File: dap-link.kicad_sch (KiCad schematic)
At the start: 46 parts, among them J1 Molex 0473460001, J2 Conn_01x05_Male, J3 SWD 10 pin 2.54mm, J4 SWD 10 pin 1.27mm, Q1 MMBT3904, U1 SC573V33RTRC, U2 STM32F103CBTx, U3 150141SV73110, Y1 8MHz

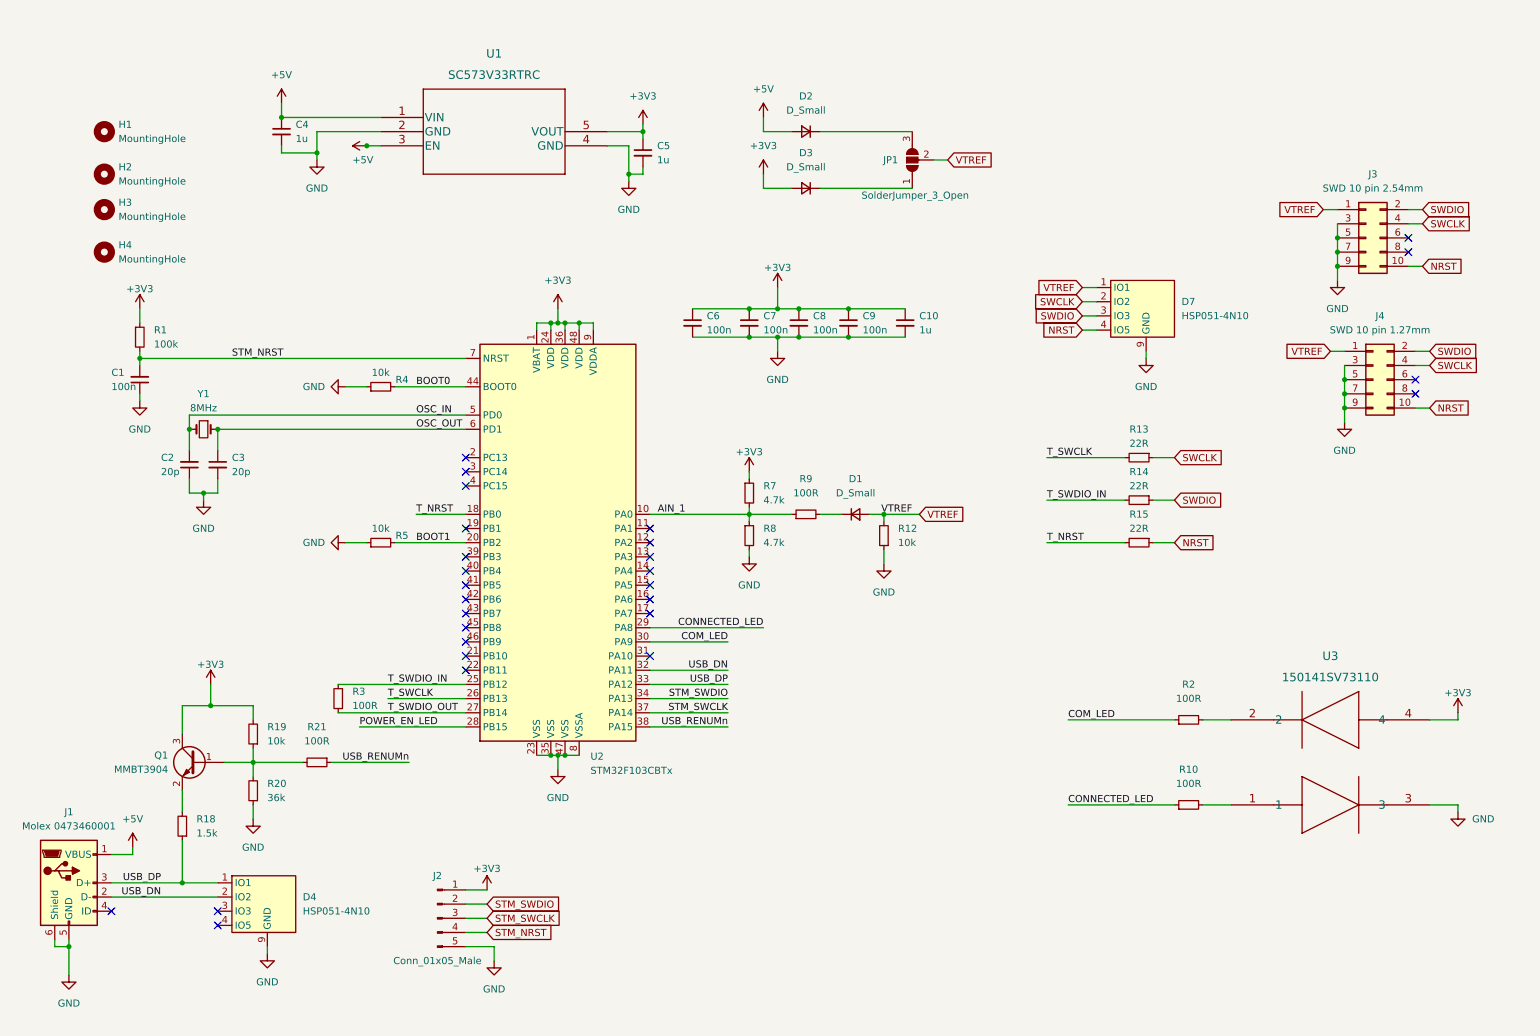
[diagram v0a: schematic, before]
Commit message: changes
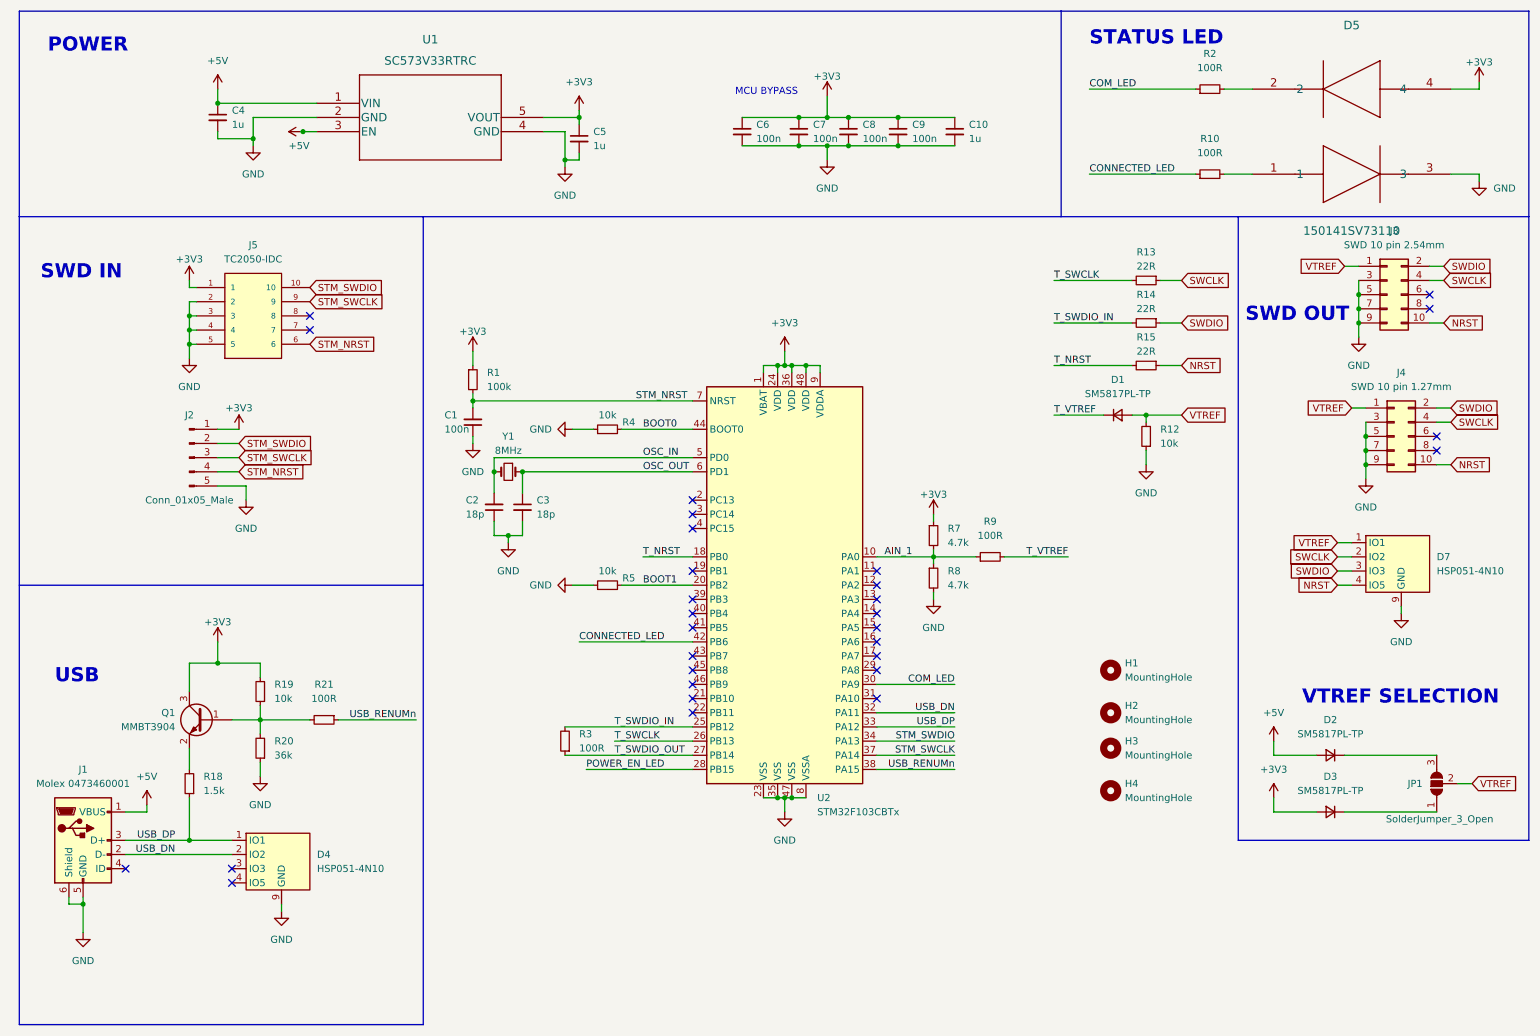
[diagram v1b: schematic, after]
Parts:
- added J5: TC2050-IDC, MyLib:TAG-CONNECT_TC2050-IDC, symbol TC2050-IDC:TC2050-IDC
- C2, C3: value 20p -> 18p
- D1, D2, D3: value D_Small -> SM5817PL-TP; footprint Diode_SMD:Nexperia_CFP3_SOD-123W -> Diode_SMD:D_SOD-123
- D4, D7: DK-PN (none) -> 497-15060-1-ND
- D5: renamed from U3; symbol dap_link_led:150141SV73110 -> 150141SV73110:150141SV73110; DK-PN (none) -> 732-13404-1-ND
- J3: DK-PN 609-4950-ND -> 1175-1621-ND
- J4: DK-PN 1175-1735-ND -> 609-4054-ND
- Q1: DK-PN (none) -> 4530-MMBT3904CT-ND
- U1: footprint SC_33RTRC_SEM -> MyLib:SC573V33RTRC; DK-PN (none) -> SC573V33RTRCCT-ND
- U2: DK-PN (none) -> 497-17380-1-ND
- Y1: DK-PN (none) -> XC2340CT-ND
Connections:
- net +3V3: now also J5.1
- net CONNECTED_LED: now also U2.42 (PB6); no longer U2.29 (PA8)
- net GND: now also J5.2, J5.3, J5.4, J5.5
- net STM_NRST: now also J5.6
- net STM_SWCLK: now also J5.9
- net STM_SWDIO: now also J5.10
- net T_VTREF: now reaches D1.1 (K), R9.2
- no-connect marks 28 -> 30
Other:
- note added: "MCU BYPASS"
- note added: "POWER"
- note added: "STATUS LED"
- note added: "SWD IN"
- note added: "SWD OUT"
- note added: "USB"
- note added: "VTREF SELECTION"
- moved on the sheet: C1, C10, C2, C3, C4, C5, C6, C7, C8, C9, D1, D2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
